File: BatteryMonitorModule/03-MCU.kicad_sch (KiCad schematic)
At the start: 17 parts, among them J3 Conn_ARM_JTAG_SWD_10, J4 USB-C, SW1 BOOT0, SW2 NRST, U1 STM32G0B1CCT6, U2 INA226AQDGSRQ1

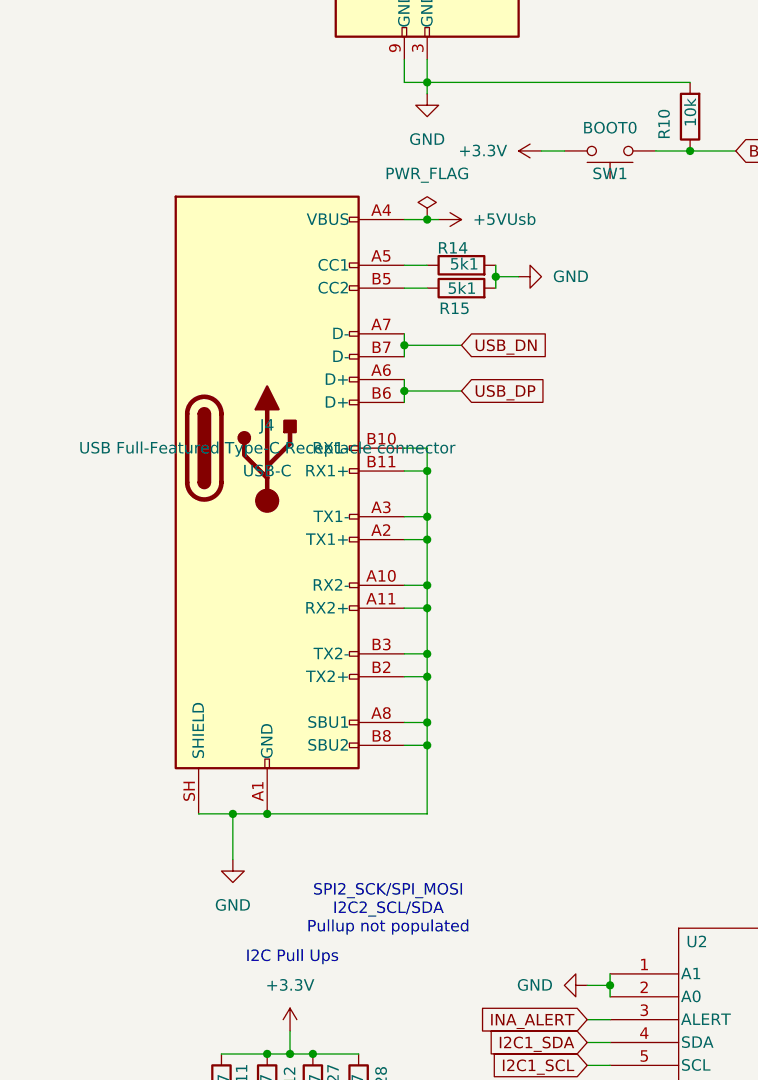
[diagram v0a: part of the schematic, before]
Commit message: design done commit
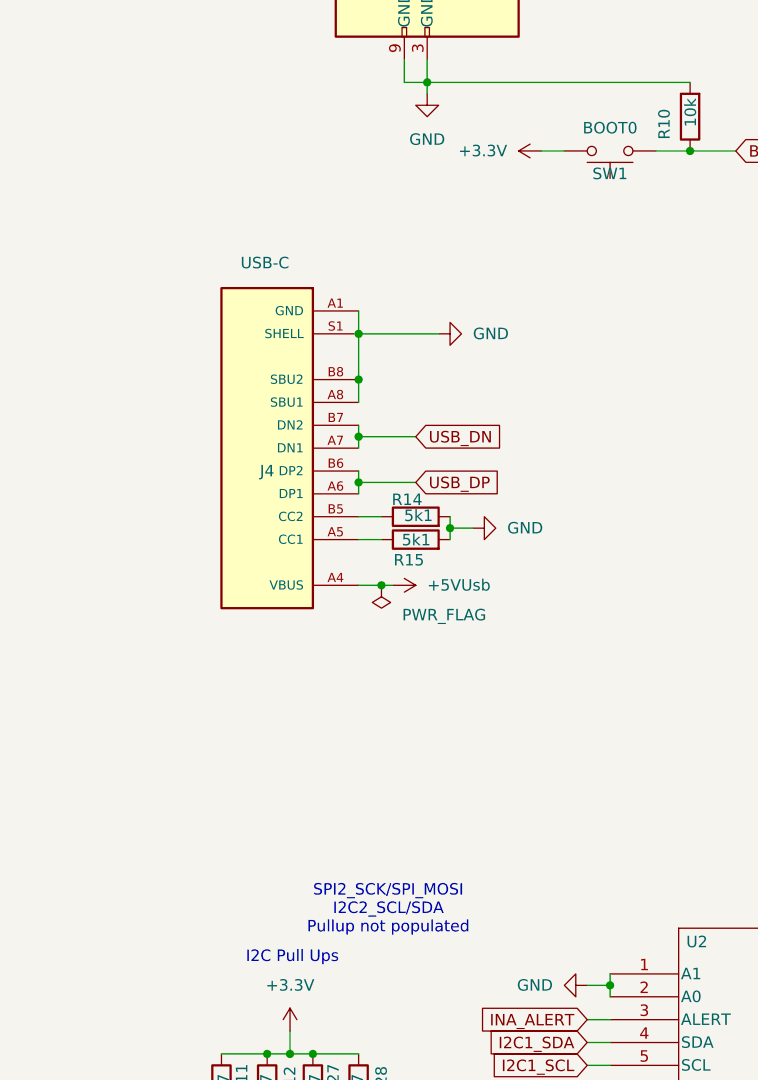
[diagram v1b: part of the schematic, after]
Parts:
- J4: footprint BatteryMonitorModule_Custom:USB4085-GF-A_GCT -> BatteryMonitorModule_Custom:GCT_USB4085-GF-A_REVA4; symbol Connector:USB_C_Receptacle -> USB4085-GF-A_REVA4:USB4085-GF-A_REVA4; Availability (none) -> In Stock; Check_prices (none) -> https://www.snapeda.com/parts/USB4085-GF-A/Global+Connector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; MANUFACTURER (none) -> Global Connector Technology; MAXIMUM_PACKAGE_HEIGHT (none) -> 3.46 mm; MF (none) -> Global Connector Technology; MP (none) -> USB4085-GF-A; PARTREV (none) -> A4; Package (none) -> None; Price (none) -> None; SNAPEDA_PN (none) -> USB4085-GF-A; STANDARDD (none) -> Manufacturer Recommendations; SnapEDA_Link (none) -> https://www.snapeda.com/parts/USB4085-GF-A/Global+Connector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
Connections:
- net GND: now also J4.S1 (SHELL), J4.S2 (SHELL), J4.S3 (SHELL), J4.S4 (SHELL); no longer J4.A10 (RX2-), J4.A11 (RX2+), J4.A2 (TX1+), J4.A3 (TX1-), J4.B10 (RX1-), J4.B11 (RX1+), J4.B2 (TX2+), J4.B3 (TX2-), J4.SH (SHIELD)
- net at R14.1: now also J4.B5 (CC2); no longer J4.A5 (CC1)
- net at R15.1: now also J4.A5 (CC1); no longer J4.B5 (CC2)
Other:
- moved on the sheet: R14, R15
